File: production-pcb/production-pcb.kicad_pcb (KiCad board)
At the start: 2 copper layers, 139.8 x 42.4 mm, 124 parts, among them J1 USB_C_Receptacle_USB2.0_14P, J2 Conn_01x04, J2 Conn_Coaxial, J3 Conn_01x04, J4 Conn_01x04, J4 Conn_01x08, J5 Conn_01x04, J5 Micro_SD_Card_Det1, J6 Conn_01x02, J6 Conn_01x05, J7 Conn_01x02, J8 Conn_01x01, J9 Conn_01x01, U1 STM32H523RCTx, U2 LR2021, U2 LSM6DSV, U3 MMC5983MA, U4 BMP384, U5 MIC5504-3.3YM5, Y1 32.768MHz, Y2 24MHz, Y3 32MHz 10pF

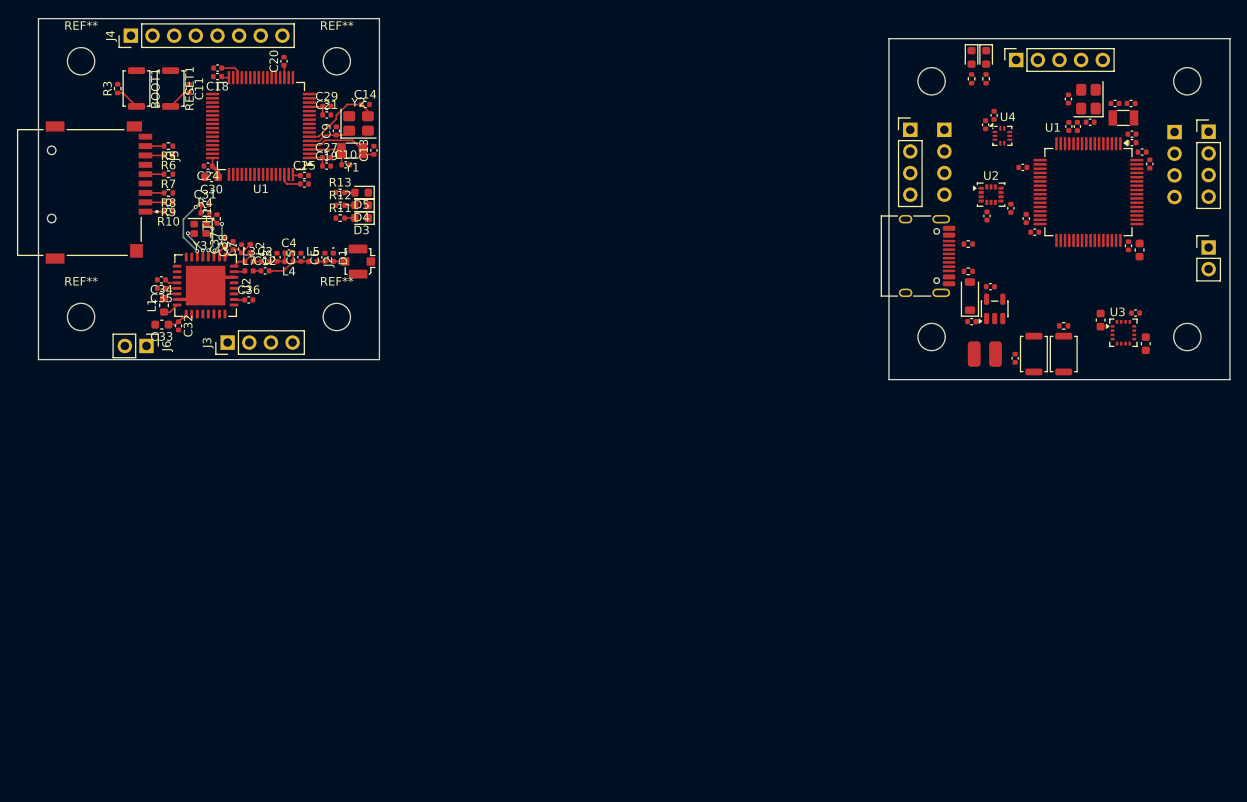
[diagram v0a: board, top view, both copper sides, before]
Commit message: started production pcb
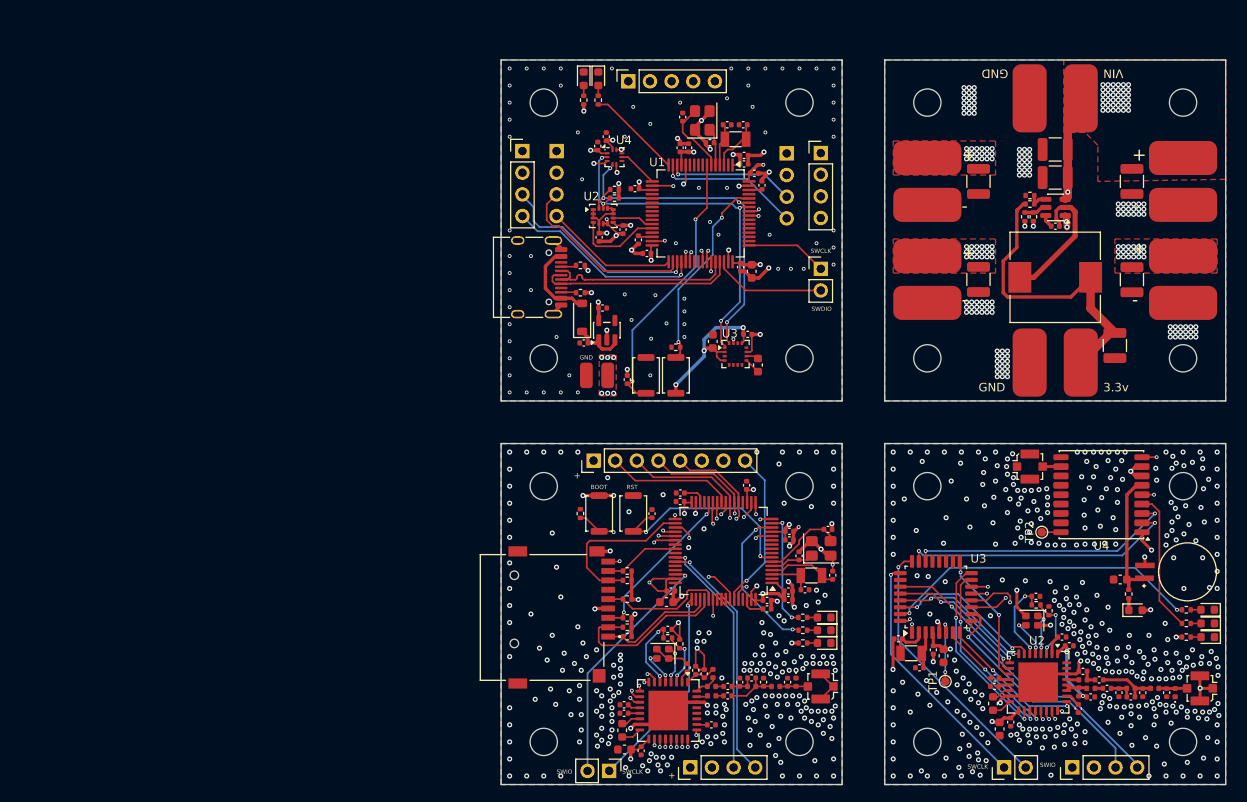
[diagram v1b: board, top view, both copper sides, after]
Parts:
- removed the BOOT1 at (62.2, 53.4)
- removed the BOOT1 at (171.0, 84.5)
- removed the C1 at (175.3, 80.5)
- removed the C10 at (178.9, 55.1)
- removed the C10 at (86.8, 62.3)
- removed the C11 at (165.3, 85.0)
- removed the C11 at (68.4, 53.4)
- removed the C12 at (77.3, 74.7)
- removed the C12 at (164.8, 67.4)
- removed the C13 at (177.0, 55.1)
- removed the C13 at (90.1, 60.6)
- removed the C14 at (171.6, 54.6)
- removed the C14 at (89.1, 55.2)
- removed the C18 at (179.0, 59.7)
- removed the C18 at (71.7, 52.0)
- removed the C19 at (84.5, 62.5)
- removed the C19 at (179.0, 58.7)
- removed the C2 at (77.3, 73.6)
- removed the C20 at (171.6, 57.8)
- removed the C20 at (79.5, 50.1)
- removed the C21 at (172.6, 57.8)
- removed the C21 at (84.5, 56.5)
- removed the C22 at (160.2, 80.7)
- removed the C23 at (162.4, 76.6)
- removed the C24 at (166.2, 62.6)
- removed the C24 at (70.6, 62.5)
- removed the C25 at (81.9, 63.5)
- removed the C25 at (167.6, 70.2)
- removed the C26 at (81.9, 64.5)
- removed the C26 at (181.1, 62.2)
- removed the C27 at (178.6, 71.8)
- removed the C27 at (84.5, 61.5)
- removed the C28 at (166.6, 68.6)
- removed the C28 at (71.7, 51.0)
- removed the C29 at (84.5, 55.5)
- removed the C29 at (180.2, 60.8)
- removed the C3 at (78.7, 73.1)
- removed the C30 at (179.9, 72.3)
- removed the C30 at (71.0, 63.8)
- removed the C31 at (70.3, 67.0)
- removed the C32 at (67.2, 81.2)
- removed the C33 at (65.2, 81.0)
- removed the C34 at (65.2, 75.8)
- removed the C35 at (65.2, 76.8)
- removed the C36 at (75.4, 78.2)
- removed the C37 at (72.6, 71.5)
- removed the C38 at (73.6, 71.8)
- removed the C4 at (162.8, 56.5)
- removed the C4 at (80.1, 72.6)
- removed the C5 at (81.5, 73.1)
- removed the C5 at (180.6, 83.3)
- removed the C6 at (161.8, 57.6)
- removed the C6 at (84.3, 73.1)
- removed the C7 at (179.4, 79.7)
- removed the C7 at (74.6, 72.1)
- removed the C8 at (162.0, 68.3)
- removed the C9 at (174.1, 57.3)
- removed the C9 at (85.7, 58.3)
- removed the D1 at (85.3, 73.1)
- removed the D1 at (160.2, 49.7)
- removed the D2 at (161.9, 49.7)
- removed the D3 at (160.0, 77.7)
- removed the D3 at (88.6, 68.5)
- removed the D4 at (88.6, 67.0)
- removed the D5 at (88.6, 65.6)
- removed the J1 at (153.5, 73.0)
- removed the J2 at (88.2, 73.6)
- removed the J2 at (153.0, 58.2)
- removed the J3 at (72.9, 83.2)
- removed the J3 at (157.0, 58.2)
- removed the J4 at (61.6, 47.1)
- removed the J4 at (184.0, 58.5)
- removed the J5 at (188.0, 58.4)
- removed the J5 at (55.5, 65.5)
- removed the J6 at (165.4, 50.0)
- removed the J6 at (63.4, 83.5)
- removed the J7 at (188.0, 72.0)
- removed the J8 at (163.0, 84.5)
- removed the J9 at (160.5, 84.5)
- removed the L1 at (65.5, 78.8)
- removed the R1 at (159.8, 71.6)
- removed the R11 at (86.1, 68.5)
- removed the R12 at (86.1, 67.0)
- removed the R13 at (161.9, 52.2)
- removed the R13 at (86.1, 65.5)
- removed the R2 at (159.8, 74.8)
- removed the R3 at (171.0, 81.2)
- removed the R3 at (60.0, 53.4)
- removed the R4 at (70.3, 68.0)
- removed the R5 at (66.0, 60.1)
- removed the REF** at (155.5, 82.5)
- removed the REF** at (55.7, 50.1)
- removed the REF** at (155.5, 52.5)
- removed the REF** at (85.7, 80.2)
- removed the REF** at (55.7, 80.2)
- removed the REF** at (185.5, 82.5)
- removed the REF** at (185.5, 52.5)
- removed the REF** at (85.7, 50.1)
- removed the RESET1 at (167.5, 84.5)
- removed the RESET1 at (66.2, 53.4)
- removed the TH1 at (71.7, 68.7)
- removed the U1 at (76.8, 57.8)
- removed the U1 at (173.9, 65.5)
- removed the U2 at (70.3, 76.5)
- removed the U2 at (162.5, 65.8)
- removed the U3 at (178.0, 82.0)
- removed the U4 at (163.8, 58.9)
- removed the Y1 at (178.0, 56.8)
- removed the Y1 at (87.5, 60.6)
- removed the Y2 at (88.3, 57.5)
- removed the Y2 at (173.9, 54.6)
- removed the Y3 at (69.7, 69.8)
- added BOOT1: SW_Push, Button_Switch_SMD:SW_Push_SPST_NO_Alps_SKRK, F.Cu at (125.5, 87.0)
- added BOOT1: SW_Push, Button_Switch_SMD:SW_Push_SPST_NO_Alps_SKRK, F.Cu at (116.5, 103.2)
- added BT1: MS621FE-FL11E, imports:BAT_MS621FE-FL11E, F.Cu at (185.5, 110.0)
- added C1: 10uF, Capacitor_SMD:C_1210_3225Metric, F.Cu at (170.0, 63.8)
- added C1: 1uF, Capacitor_SMD:C_0603_1608Metric, F.Cu at (129.8, 83.0)
- added C10: 15pF, Capacitor_SMD:C_0402_1005Metric, F.Cu at (140.7, 112.2)
- added C10: 7.5pF, Capacitor_SMD:C_0402_1005Metric, F.Cu at (177.5, 124.2)
- added C10: 10uF, Capacitor_SMD:C_1210_3225Metric, F.Cu at (161.0, 75.8)
- added C10: 15pF, Capacitor_SMD:C_0402_1005Metric, F.Cu at (133.4, 57.6)
- added C11: 100nF, Capacitor_SMD:C_0402_1005Metric, F.Cu at (119.8, 87.5)
- added C11: 100nF, Capacitor_SMD:C_0402_1005Metric, F.Cu at (122.7, 103.2)
- added C11: 1.8pF, Capacitor_SMD:C_0402_1005Metric, F.Cu at (178.9, 124.7)
- added C12: 18pF, Capacitor_SMD:C_0402_1005Metric, F.Cu at (131.6, 124.6)
- added C12: 100nF, Capacitor_SMD:C_0402_1005Metric, F.Cu at (119.3, 69.9)
- added C12: 10uF, Capacitor_SMD:C_1210_3225Metric, F.Cu at (179.0, 64.2)
- added C13: 15pF, Capacitor_SMD:C_0402_1005Metric, F.Cu at (143.9, 110.5)
- added C13: 18pF, Capacitor_SMD:C_0402_1005Metric, F.Cu at (175.2, 122.7)
- added C13: 15pF, Capacitor_SMD:C_0402_1005Metric, F.Cu at (131.5, 57.6)
- added C14: 10uF, Capacitor_SMD:C_1210_3225Metric, F.Cu at (179.0, 75.8)
- added C14: 18pF, Capacitor_SMD:C_0402_1005Metric, F.Cu at (143.3, 105.1)
- added C14: 3.9pF, Capacitor_SMD:C_0402_1005Metric, F.Cu at (180.3, 124.2)
- added C14: 18pF, Capacitor_SMD:C_0402_1005Metric, F.Cu at (126.3, 56.7)
- added C15: 1.8pF, Capacitor_SMD:C_0402_1005Metric, F.Cu at (183.1, 124.2)
- added C16: 2.2pF, Capacitor_SMD:C_0402_1005Metric, F.Cu at (173.3, 121.7)
- added C17: 1uF, Capacitor_SMD:C_0603_1608Metric, F.Cu at (177.6, 111.0)
- added C18: 100nF, Capacitor_SMD:C_0402_1005Metric, F.Cu at (126.0, 101.8)
- added C18: 100nF, Capacitor_SMD:C_0402_1005Metric, F.Cu at (155.7, 119.2)
- added C18: 100nF, Capacitor_SMD:C_0402_1005Metric, F.Cu at (133.5, 62.2)
- added C19: 4.7uF, Capacitor_SMD:C_0603_1608Metric, F.Cu at (156.9, 119.9)
- added C19: 1uF, Capacitor_SMD:C_0402_1005Metric, F.Cu at (133.5, 61.2)
- added C19: 1uF, Capacitor_SMD:C_0402_1005Metric, F.Cu at (138.7, 113.3)
- added C2: 10uF, Capacitor_SMD:C_1210_3225Metric, F.Cu at (170.0, 60.5)
- added C2: 6.8pF, Capacitor_SMD:C_0402_1005Metric, F.Cu at (131.6, 123.5)
- added C20: 100nF, Capacitor_SMD:C_0402_1005Metric, F.Cu at (126.0, 60.3)
- added C20: 100nF, Capacitor_SMD:C_0402_1005Metric, F.Cu at (133.8, 99.9)
- added C21: 1uF, Capacitor_SMD:C_0402_1005Metric, F.Cu at (138.8, 106.3)
- added C21: 1uF, Capacitor_SMD:C_0402_1005Metric, F.Cu at (127.0, 60.3)
- added C22: 1uF, Capacitor_SMD:C_0402_1005Metric, F.Cu at (114.7, 83.2)
- added C22: 47pF, Capacitor_SMD:C_0402_1005Metric, F.Cu at (151.6, 117.9)
- added C23: 1uF, Capacitor_SMD:C_0402_1005Metric, F.Cu at (116.9, 79.1)
- added C23: 47pF, Capacitor_SMD:C_0402_1005Metric, F.Cu at (154.1, 121.3)
- added C24: 100nF, Capacitor_SMD:C_0402_1005Metric, F.Cu at (124.9, 112.3)
- added C24: 100nF, Capacitor_SMD:C_0402_1005Metric, F.Cu at (120.7, 65.1)
- added C25: 100nF, Capacitor_SMD:C_0402_1005Metric, F.Cu at (136.2, 113.4)
- added C25: 100nF, Capacitor_SMD:C_0402_1005Metric, F.Cu at (122.1, 72.7)
- added C26: 2.2uF, Capacitor_SMD:C_0402_1005Metric, F.Cu at (136.2, 114.4)
- added C26: 2.2uF, Capacitor_SMD:C_0402_1005Metric, F.Cu at (135.6, 64.7)
- added C27: 100nF, Capacitor_SMD:C_0402_1005Metric, F.Cu at (138.7, 112.3)
- added C27: 100nF, Capacitor_SMD:C_0402_1005Metric, F.Cu at (133.1, 74.3)
- added C28: 2.2uF, Capacitor_SMD:C_0402_1005Metric, F.Cu at (126.0, 100.8)
- added C28: 2.2uF, Capacitor_SMD:C_0402_1005Metric, F.Cu at (121.1, 71.1)
- added C29: 100nF, Capacitor_SMD:C_0402_1005Metric, F.Cu at (138.8, 105.3)
- added C29: 100nF, Capacitor_SMD:C_0402_1005Metric, F.Cu at (134.7, 63.3)
- added C3: 2.7pF, Capacitor_SMD:C_0402_1005Metric, F.Cu at (133.0, 123.0)
- added C3: 47uF, Capacitor_SMD:C_1210_3225Metric, F.Cu at (177.0, 83.5)
- added C30: 4.7uF, Capacitor_SMD:C_0603_1608Metric, F.Cu at (134.4, 74.8)
- added C30: 4.7uF, Capacitor_SMD:C_0603_1608Metric, F.Cu at (124.4, 113.6)
- added C31: 100nF, Capacitor_SMD:C_0402_1005Metric, F.Cu at (124.5, 116.8)
- added C31: 100nF, Capacitor_SMD:C_0402_1005Metric, F.Cu at (167.7, 112.9)
- added C32: 100nF, Capacitor_SMD:C_0402_1005Metric, F.Cu at (121.4, 131.0)
- added C32: 100nF, Capacitor_SMD:C_0402_1005Metric, F.Cu at (164.8, 127.7)
- added C33: 4.7uF, Capacitor_SMD:C_0603_1608Metric, F.Cu at (119.5, 130.9)
- added C33: 4.7uF, Capacitor_SMD:C_0603_1608Metric, F.Cu at (163.5, 128.5)
- added C34: 1uF, Capacitor_SMD:C_0402_1005Metric, F.Cu at (162.9, 122.5)
- added C34: 1uF, Capacitor_SMD:C_0402_1005Metric, F.Cu at (119.4, 125.6)
- added C35: 2.2uF, Capacitor_SMD:C_0402_1005Metric, F.Cu at (162.9, 123.5)
- added C35: 2.2uF, Capacitor_SMD:C_0402_1005Metric, F.Cu at (119.4, 126.6)
- added C36: 1uF, Capacitor_SMD:C_0402_1005Metric, F.Cu at (129.7, 128.0)
- added C36: 1uF, Capacitor_SMD:C_0402_1005Metric, F.Cu at (172.7, 126.1)
- added C37: 2.2uF, Capacitor_SMD:C_0402_1005Metric, F.Cu at (126.8, 121.3)
- added C37: 2.2uF, Capacitor_SMD:C_0402_1005Metric, F.Cu at (170.8, 117.7)
- added C38: 1nF, Capacitor_SMD:C_0402_1005Metric, F.Cu at (127.8, 121.6)
- added C38: 1nF, Capacitor_SMD:C_0402_1005Metric, F.Cu at (171.7, 118.7)
- added C4: 1.1pF, Capacitor_SMD:C_0402_1005Metric, F.Cu at (134.4, 122.5)
- added C4: 100nF, Capacitor_SMD:C_0402_1005Metric, F.Cu at (117.3, 59.0)
- added C4: 100nF, Capacitor_SMD:C_0402_1005Metric, F.Cu at (170.0, 69.5)
- added C5: 1.2pF, Capacitor_SMD:C_0402_1005Metric, F.Cu at (135.8, 123.0)
- added C5: 10uF, Capacitor_SMD:C_0603_1608Metric, F.Cu at (135.1, 85.8)
- added C6: 100nF, Capacitor_SMD:C_0402_1005Metric, F.Cu at (116.3, 60.1)
- added C6: 2pF, Capacitor_SMD:C_0402_1005Metric, F.Cu at (138.6, 123.0)
- added C7: 100nF, Capacitor_SMD:C_0402_1005Metric, F.Cu at (133.9, 82.2)
- added C7: 47pF, Capacitor_SMD:C_0402_1005Metric, F.Cu at (128.8, 122.0)
- added C8: 100nF, Capacitor_SMD:C_0402_1005Metric, F.Cu at (116.5, 70.8)
- added C8: 47pF, Capacitor_SMD:C_0402_1005Metric, F.Cu at (174.2, 124.7)
- added C8: 10uF, Capacitor_SMD:C_1210_3225Metric, F.Cu at (161.0, 64.2)
- added C9: 22pF, Capacitor_SMD:C_0402_1005Metric, F.Cu at (176.1, 123.7)
- added C9: 18pF, Capacitor_SMD:C_0402_1005Metric, F.Cu at (139.9, 108.2)
- added C9: 18pF, Capacitor_SMD:C_0402_1005Metric, F.Cu at (129.5, 59.7)
- added D1: D_TVS, Diode_SMD:D_0402_1005Metric, F.Cu at (139.6, 123.0)
- added D1: LED, LED_SMD:LED_0603_1608Metric, F.Cu at (114.7, 52.2)
- added D2: D_TVS, Diode_SMD:D_0402_1005Metric, F.Cu at (184.1, 124.2)
- added D2: LED, LED_SMD:LED_0603_1608Metric, F.Cu at (116.4, 52.2)
- added D3: D_Schottky, Diode_SMD:D_0603_1608Metric, F.Cu at (179.4, 114.5)
- added D3: LED, LED_SMD:LED_0603_1608Metric, F.Cu at (142.9, 118.4)
- added D3: D_Schottky, Diode_SMD:D_SOD-123, F.Cu at (114.5, 80.2)
- added D4: LED, LED_SMD:LED_0603_1608Metric, F.Cu at (142.9, 116.9)
- added D4: LED, LED_SMD:LED_0603_1608Metric, F.Cu at (187.9, 117.7)
- added D5: LED, LED_SMD:LED_0603_1608Metric, F.Cu at (142.9, 115.4)
- added D5: LED, LED_SMD:LED_0603_1608Metric, F.Cu at (187.9, 116.1)
- added D6: LED, LED_SMD:LED_0603_1608Metric, F.Cu at (187.9, 114.5)
- added J1: USB_C_Receptacle_USB2.0_14P, Connector_USB:USB_C_Receptacle_HRO_TYPE-C-31-M-12, F.Cu at (108.0, 75.5)
- added J1: Conn_01x01, Connector_Wire:SolderWirePad_1x01_SMD_4x8mm, F.Cu at (173.0, 54.5)
- added J10: Conn_01x01, Connector_Wire:SolderWirePad_1x01_SMD_4x8mm, F.Cu at (185.0, 67.0)
- added J11: Conn_01x01, Connector_Wire:SolderWirePad_1x01_SMD_4x8mm, F.Cu at (185.0, 73.0)
- added J12: Conn_01x01, Connector_Wire:SolderWirePad_1x01_SMD_4x8mm, F.Cu at (185.0, 78.5)
- added J2: Conn_Coaxial, Connector_Coaxial:U.FL_Molex_MCRF_73412-0110_Vertical, F.Cu at (187.0, 123.7)
- added J2: Conn_01x01, Connector_Wire:SolderWirePad_1x01_SMD_4x8mm, F.Cu at (167.0, 54.5)
- added J2: Conn_Coaxial, Connector_Coaxial:U.FL_Molex_MCRF_73412-0110_Vertical, F.Cu at (142.5, 123.5)
- added J2: Conn_01x04, Connector_PinHeader_2.54mm:PinHeader_1x04_P2.54mm_Vertical, F.Cu at (107.5, 60.7)
- added J3: Conn_01x01, Connector_Wire:SolderWirePad_1x01_SMD_4x8mm, F.Cu at (173.0, 85.5)
- added J3: Conn_01x04, Connector_PinHeader_2.54mm:PinHeader_1x04_P2.54mm_Vertical, F.Cu at (127.2, 133.0)
- added J3: Conn_01x04, Connector_PinHeader_2.54mm:PinHeader_1x04_P2.54mm_Vertical, F.Cu at (172.0, 133.0)
- added J3: Conn_01x04, Connector_PinHeader_2.54mm:PinHeader_1x04_P2.54mm_Vertical, B.Cu at (111.5, 60.7)
- added J4: Conn_01x08, Connector_PinHeader_2.54mm:PinHeader_1x08_P2.54mm_Vertical, F.Cu at (115.8, 97.0)
- added J4: Conn_01x02, Connector_PinHeader_2.54mm:PinHeader_1x02_P2.54mm_Vertical, F.Cu at (164.0, 133.0)
- added J4: Conn_01x01, Connector_Wire:SolderWirePad_1x01_SMD_4x8mm, F.Cu at (167.0, 85.5)
- added J4: Conn_01x04, Connector_PinHeader_2.54mm:PinHeader_1x04_P2.54mm_Vertical, B.Cu at (138.5, 61.0)
- added J5: Micro_SD_Card_Det1, camera-controller:CUI_MSD-4-A, F.Cu at (109.8, 115.4)
- added J5: Conn_01x01, Connector_Wire:SolderWirePad_1x01_SMD_4x8mm, F.Cu at (155.0, 61.5)
- added J5: Conn_01x04, Connector_PinHeader_2.54mm:PinHeader_1x04_P2.54mm_Vertical, F.Cu at (142.5, 60.9)
- added J5: Conn_Coaxial, Connector_Coaxial:U.FL_Molex_MCRF_73412-0110_Vertical, F.Cu at (167.0, 97.7)
- added J6: Conn_01x02, Connector_PinHeader_2.54mm:PinHeader_1x02_P2.54mm_Vertical, F.Cu at (117.7, 133.4)
- added J6: Conn_01x05, Connector_PinSocket_2.54mm:PinSocket_1x05_P2.54mm_Vertical, F.Cu at (119.9, 52.5)
- added J6: Conn_01x01, Connector_Wire:SolderWirePad_1x01_SMD_4x8mm, F.Cu at (155.0, 67.0)
- added J7: Conn_01x02, Connector_PinHeader_2.54mm:PinHeader_1x02_P2.54mm_Vertical, F.Cu at (142.5, 74.5)
- added J7: Conn_01x01, Connector_Wire:SolderWirePad_1x01_SMD_4x8mm, F.Cu at (155.0, 73.0)
- added J8: Conn_01x01, Connector_Wire:SolderWirePad_1x01_SMD_4x8mm, F.Cu at (155.0, 78.5)
- added J8: Conn_01x01, Connector_Wire:SolderWirePad_1x01_SMD_1.5x3mm, F.Cu at (117.5, 87.0)
- added J9: Conn_01x01, Connector_Wire:SolderWirePad_1x01_SMD_4x8mm, F.Cu at (185.0, 61.5)
- added J9: Conn_01x01, Connector_Wire:SolderWirePad_1x01_SMD_1.5x3mm, F.Cu at (115.0, 87.0)
- added L1: 2.2uH, Inductor_SMD:L_0603_1608Metric, F.Cu at (119.2, 128.6)
- added L1: 10uH, Inductor_SMD:L_10.4x10.4_H4.8, F.Cu at (170.0, 75.5)
- added L1: 2.2uH, Inductor_SMD:L_0603_1608Metric, F.Cu at (162.7, 125.5)
- added L10: 3.9nH, Inductor_SMD:L_0402_1005Metric, F.Cu at (178.9, 123.7)
- added L11: 7.5nH, Inductor_SMD:L_0402_1005Metric, F.Cu at (181.7, 123.7)
- added L6: 12nH, Inductor_SMD:L_0402_1005Metric, F.Cu at (172.8, 124.1)
- added L8: 4.7nH, Inductor_SMD:L_0402_1005Metric, F.Cu at (174.2, 123.7)
- added L9: 24nH, Inductor_SMD:L_0402_1005Metric, F.Cu at (173.3, 122.7)
- added R1: 5.1K, Resistor_SMD:R_0402_1005Metric, F.Cu at (114.3, 74.1)
- added R1: 100K, Resistor_SMD:R_0402_1005Metric, F.Cu at (167.0, 66.9)
- added R11: 1.2K, Resistor_SMD:R_0402_1005Metric, F.Cu at (140.4, 118.4)
- added R11: 1.2K, Resistor_SMD:R_0402_1005Metric, F.Cu at (185.4, 117.7)
- added R12: 1.2K, Resistor_SMD:R_0402_1005Metric, F.Cu at (185.4, 116.1)
- added R12: 1.2K, Resistor_SMD:R_0402_1005Metric, F.Cu at (140.4, 116.9)
- added R13: 1.2K, Resistor_SMD:R_0402_1005Metric, F.Cu at (185.4, 114.5)
- added R13: 1.2K, Resistor_SMD:R_0402_1005Metric, F.Cu at (140.4, 115.4)
- added R13: 1K, Resistor_SMD:R_0402_1005Metric, F.Cu at (116.4, 54.7)
- added R2: 5.1K, Resistor_SMD:R_0402_1005Metric, F.Cu at (114.3, 77.3)
- added R2: 22K, Resistor_SMD:R_0402_1005Metric, F.Cu at (167.0, 65.9)
- added R3: 1K, Resistor_SMD:R_0402_1005Metric, F.Cu at (178.6, 112.7)
- added R3: 10K, Resistor_SMD:R_0402_1005Metric, F.Cu at (114.3, 103.2)
- added R3: 100K, Resistor_SMD:R_0402_1005Metric, F.Cu at (167.4, 68.4)
- added R3: 10K, Resistor_SMD:R_0402_1005Metric, F.Cu at (125.5, 83.7)
- added R4: 120K, Resistor_SMD:R_0402_1005Metric, F.Cu at (124.5, 117.8)
- added R4: 33.2K, Resistor_SMD:R_0402_1005Metric, F.Cu at (166.4, 68.4)
- added R4: 120K, Resistor_SMD:R_0402_1005Metric, F.Cu at (167.8, 113.9)
- added R4: 1.2K, Resistor_SMD:R_0402_1005Metric, F.Cu at (118.3, 66.2)
- added R5: 10K, Resistor_SMD:R_0402_1005Metric, F.Cu at (119.8, 110.0)
- added R5: 1.2K, Resistor_SMD:R_0402_1005Metric, F.Cu at (118.3, 65.2)
- added REF**: MountingHole_3.2mm_M3, MountingHole:MountingHole_3.2mm_M3, F.Cu at (185.0, 55.0)
- added REF**: MountingHole_3.2mm_M3, MountingHole:MountingHole_3.2mm_M3, F.Cu at (185.0, 100.0)
- added REF**: MountingHole_3.2mm_M3, MountingHole:MountingHole_3.2mm_M3, F.Cu at (185.0, 85.0)
- added REF**: MountingHole_3.2mm_M3, MountingHole:MountingHole_3.2mm_M3, F.Cu at (155.0, 55.0)
- added REF**: MountingHole_3.2mm_M3, MountingHole:MountingHole_3.2mm_M3, F.Cu at (185.0, 130.0)
- added REF**: MountingHole_3.2mm_M3, MountingHole:MountingHole_3.2mm_M3, F.Cu at (155.0, 85.0)
- added REF**: MountingHole_3.2mm_M3, MountingHole:MountingHole_3.2mm_M3, F.Cu at (155.0, 130.0)
- added REF**: MountingHole_3.2mm_M3, MountingHole:MountingHole_3.2mm_M3, F.Cu at (140.0, 55.0)
- added REF**: MountingHole_3.2mm_M3, MountingHole:MountingHole_3.2mm_M3, F.Cu at (110.0, 100.0)
- added REF**: MountingHole_3.2mm_M3, MountingHole:MountingHole_3.2mm_M3, F.Cu at (155.0, 100.0)
- added REF**: MountingHole_3.2mm_M3, MountingHole:MountingHole_3.2mm_M3, F.Cu at (110.0, 130.0)
- added REF**: MountingHole_3.2mm_M3, MountingHole:MountingHole_3.2mm_M3, F.Cu at (140.0, 85.0)
- added REF**: MountingHole_3.2mm_M3, MountingHole:MountingHole_3.2mm_M3, F.Cu at (110.0, 55.0)
- added REF**: MountingHole_3.2mm_M3, MountingHole:MountingHole_3.2mm_M3, F.Cu at (110.0, 85.0)
- added REF**: MountingHole_3.2mm_M3, MountingHole:MountingHole_3.2mm_M3, F.Cu at (140.0, 100.0)
- added REF**: MountingHole_3.2mm_M3, MountingHole:MountingHole_3.2mm_M3, F.Cu at (140.0, 130.0)
- added RESET1: SW_Push, Button_Switch_SMD:SW_Push_SPST_NO_Alps_SKRK, F.Cu at (122.0, 87.0)
- added RESET1: SW_Push, Button_Switch_SMD:SW_Push_SPST_NO_Alps_SKRK, F.Cu at (120.5, 103.2)
- added TH1: ERT-J0ER104F, Resistor_SMD:R_0402_1005Metric, F.Cu at (169.3, 114.6)
- added TH1: ERT-J0ER104F, Resistor_SMD:R_0402_1005Metric, F.Cu at (125.9, 118.5)
- added TP1: TestPoint, TestPoint:TestPoint_Pad_D1.0mm, F.Cu at (157.1, 122.9)
- added TP2: TestPoint, TestPoint:TestPoint_Pad_D1.0mm, F.Cu at (168.4, 105.4)
- added U1: STM32H523RCTx, Package_QFP:LQFP-64_10x10mm_P0.5mm, F.Cu at (131.1, 107.6)
- added U1: TPS54308, Package_TO_SOT_SMD:SOT-23-6, F.Cu at (170.0, 67.3)
- added U1: STM32H523RCTx, Package_QFP:LQFP-64_10x10mm_P0.5mm, F.Cu at (128.4, 68.0)
- added U2: LR2021, Package_DFN_QFN:QFN-32-1EP_7x7mm_P0.65mm_EP4.65x4.65mm, F.Cu at (124.6, 126.3)
- added U2: LR2021, Package_DFN_QFN:QFN-32-1EP_7x7mm_P0.65mm_EP4.65x4.65mm, F.Cu at (168.0, 123.0)
- added U2: LSM6DSV, Package_LGA:LGA-14_3x2.5mm_P0.5mm_LayoutBorder3x4y, F.Cu at (117.0, 68.3)
- added U3: MMC5983MA, Package_LGA:LGA-16_3x3mm_P0.5mm, F.Cu at (132.5, 84.5)
- added U3: STM32G030K8Tx, Package_QFP:LQFP-32_7x7mm_P0.8mm, F.Cu at (156.0, 113.0)
- added U4: MAX-M10S, RF_GPS:ublox_MAX, F.Cu at (175.4, 101.0)
- added U4: BMP384, Package_LGA:Rohm_MLGA010V020A_LGA-10_2x2mm_P0.45mm_LayoutBorder2x3y, F.Cu at (118.3, 61.4)
- added Y1: 32.768MHz, Crystal:Crystal_SMD_3215-2Pin_3.2x1.5mm, F.Cu at (132.5, 59.3)
- added Y1: 32.768KHz, Crystal:Crystal_SMD_3215-2Pin_3.2x1.5mm, F.Cu at (153.1, 119.6)
- added Y1: 32.768MHz, Crystal:Crystal_SMD_3215-2Pin_3.2x1.5mm, F.Cu at (141.4, 110.5)
- added Y2: 24MHz, Crystal:Crystal_SMD_3225-4Pin_3.2x2.5mm, F.Cu at (142.6, 107.3)
- added Y2: 24MHz, Crystal:Crystal_SMD_3225-4Pin_3.2x2.5mm, F.Cu at (128.6, 57.1)
- added Y3: 32MHz 10pF, Crystal:Crystal_SMD_2016-4Pin_2.0x1.6mm, F.Cu at (167.3, 115.8)
- added Y3: 32MHz 10pF, Crystal:Crystal_SMD_2016-4Pin_2.0x1.6mm, F.Cu at (124.0, 119.7)
- moved L3 73.7 mm to (129.7, 123.5)
- moved L4 73.7 mm to (134.4, 123.5)
- moved L5 73.7 mm to (137.2, 123.5)
- moved L2 73.7 mm to (129.8, 122.0)
- moved L7 73.7 mm to (129.7, 124.6)
- moved R10 73.4 mm to (119.8, 117.7)
- moved R6 73.4 mm to (119.8, 111.0)
- moved R7 73.4 mm to (119.8, 113.2)
- moved R8 73.4 mm to (119.8, 115.5)
- moved R9 73.4 mm to (119.8, 116.5)
- moved R15 45.6 mm to (114.7, 54.7)
- moved U5 45.6 mm to (117.4, 81.7)
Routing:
- net GND: track 7.75 -> 147.6 mm, vias 0 -> 805
- net +3.3V: track 13.6 -> 136.7 mm, vias 0 -> 39
- net /SWDIO: track 0.00 -> 73.7 mm, vias 0 -> 2
- net /SCL: track 0.00 -> 69.7 mm, vias 0 -> 5
- net /MOSI: track 0.00 -> 67.2 mm, vias 0 -> 4
- net /MISO: track 0.00 -> 65.1 mm, vias 0 -> 4
- net /SCK: track 0.00 -> 64.7 mm, vias 0 -> 4
- net /SWCLK: track 0.00 -> 63.1 mm, vias 0 -> 2
- net /SDA: track 0.00 -> 61.2 mm, vias 0 -> 5
- net /UART_RX: track 0.00 -> 59.2 mm, vias 0 -> 2
- net /UART_TX: track 0.00 -> 56.9 mm, vias 0 -> 2
- net /LR_D5: track 0.00 -> 56.4 mm, vias 0 -> 4
- net /LR_D6: track 0.00 -> 55.0 mm, vias 0 -> 4
- net /STM32_RST: track 2.86 -> 57.1 mm, vias 0 -> 4
- net /LR_STAT: track 0.00 -> 51.3 mm, vias 0 -> 4
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- added copper zone on F.Cu, net +3.3V
- added copper zone on In1.Cu, net +3.3V
- added copper zone on B.Cu, net GND
- added copper zone on F.Cu, net GND
- added copper zone on In2.Cu, net GND
- added copper zone on F.Cu, net VBUS
- added copper zone on In1.Cu, net VBUS
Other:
- board size 139.8 x 42.4 mm -> 85 x 85 mm
- copper layers 2 -> 4
- board text added: "+"
- board text added: "-"
- board text added: "3.3v"
- board text added: "BOOT"
- board text added: "GND"
- board text added: "RST"
- board text added: "SWCLK"
- board text added: "SWDIO"
- board text added: "SWIO"
- board text added: "VIN"

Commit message: added production files
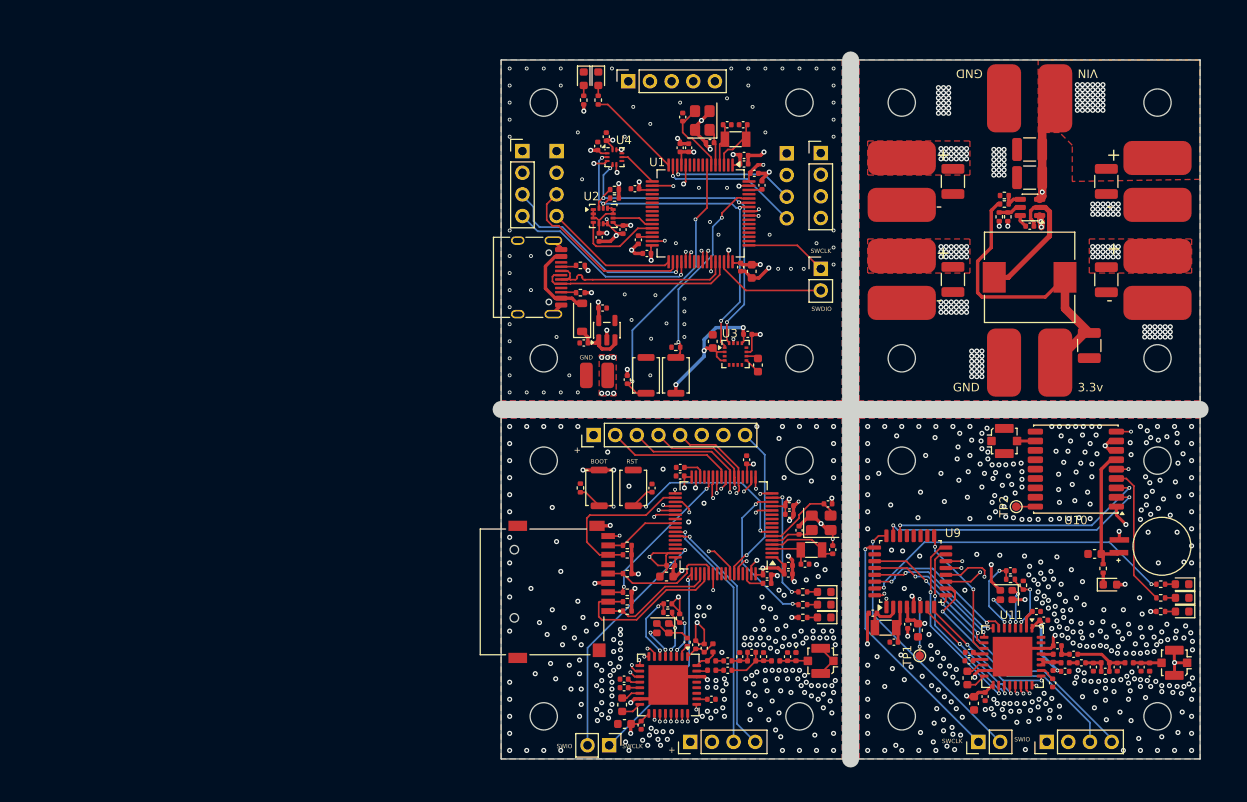
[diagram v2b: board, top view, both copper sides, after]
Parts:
- moved BT1 4.24 mm to (182.5, 107.0)
- moved C65 4.24 mm to (152.7, 116.2)
- moved C66 4.24 mm to (153.9, 116.9)
- moved C67 4.24 mm to (148.6, 114.9)
- moved C68 4.24 mm to (151.1, 118.3)
- moved C69 4.24 mm to (164.7, 109.9)
- moved C70 4.24 mm to (161.8, 124.7)
- moved C72 4.24 mm to (167.8, 114.7)
- moved C73 4.24 mm to (159.9, 120.5)
- moved C74 4.24 mm to (174.6, 108.0)
- moved C75 4.24 mm to (169.7, 123.1)
- moved C76 4.24 mm to (159.9, 119.5)
- moved C77 4.24 mm to (168.7, 115.7)
- moved C78 4.24 mm to (171.2, 121.7)
- moved C79 4.24 mm to (173.1, 120.7)
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- renumbered BOOT1 to BOOT2, C8 to C15, C10 to C16, C12 to C17, C1 to C3, C14 to C31, C4 to C32, C3 to C33, C14 to C34, C10 to C35, C13 to C36, C9 to C37, C28 to C38, C26 to C39, C29 to C40, C21 to C41, C27 to C42, C11 to C43, C19 to C44, C25 to C45, C24 to C46, C18 to C47, C20 to C48, C30 to C49, C31 to C50, C7 to C51, C2 to C52, C32 to C53, C3 to C54, C33 to C55, C4 to C56, C12 to C57, C37 to C58, C5 to C59, C35 to C60, C36 to C61, C6 to C62, C34 to C63, C38 to C64, C18 to C65, C19 to C66, C22 to C67, C23 to C68, C31 to C69, C32 to C70, C33 to C71, C37 to C72, C35 to C73, C17 to C74, C36 to C75, C34 to C76, C38 to C77, C8 to C78, C9 to C79, C16 to C80, C10 to C81, C11 to C82, C13 to C83, C14 to C84, C15 to C85, D5 to D10, D6 to D11, D2 to D12, D3 to D4, D4 to D5, D5 to D6, D1 to D7, D3 to D8, D4 to D9, J1 to J10, J2 to J11, J5 to J12, J6 to J13, J7 to J14, J8 to J15, J9 to J16, J10 to J17, J11 to J18, J12 to J19, J3 to J20, J4 to J21, J3 to J22, J4 to J23, J6 to J24, J5 to J25, J2 to J26, J5 to J29, J2 to J30, L8 to L10, L9 to L11, L10 to L12, L11 to L13, L1 to L6, L1 to L8, L6 to L9, R9 to R11, R8 to R12, R7 to R14, R6 to R16, R5 to R17, R11 to R18, R12 to R19, R13 to R20, R3 to R21, R4 to R22, R4 to R23, R3 to R24, R11 to R25, R12 to R26, R13 to R27, R3 to R6, R4 to R7, R1 to R8, R2 to R9, RESET1 to RESET2, TH1 to TH2, U4 to U10, U2 to U11, U1 to U6, U1 to U7, U2 to U8, U3 to U9, Y1 to Y3, Y2 to Y4, Y3 to Y5, Y1 to Y6, Y3 to Y7
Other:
- board size 85 x 85 mm -> 82 x 82 mm
